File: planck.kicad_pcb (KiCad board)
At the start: 2 copper layers, 113 x 75 mm, 84 parts, among them J1 USB_C_U262-161N-4BVC11, J2 USB_C_U262-161N-4BVC11, SW1 SW_Cherry_MX_1.00u, SW10 SW_Cherry_MX_1.00u, SW11 SW_Cherry_MX_1.00u, SW12 SW_Cherry_MX_1.00u, SW13 SW_Cherry_MX_1.00u, SW14 SW_Cherry_MX_1.00u, SW15 SW_Cherry_MX_1.00u, SW16 SW_Cherry_MX_1.00u, SW17 SW_Cherry_MX_1.00u, SW18 SW_Cherry_MX_1.00u, SW19 SW_Cherry_MX_1.00u, SW2 SW_Cherry_MX_1.00u, SW20 SW_Cherry_MX_1.00u, SW21 SW_Cherry_MX_1.00u, SW22 SW_Cherry_MX_1.00u, SW23 SW_Cherry_MX_1.00u, SW24 SW_Cherry_MX_1.00u, SW25 SW_Push, SW3 SW_Cherry_MX_1.00u, SW4 SW_Cherry_MX_1.00u, SW5 SW_Cherry_MX_1.00u, SW6 SW_Cherry_MX_1.00u, SW7 SW_Cherry_MX_1.00u, SW8 SW_Cherry_MX_1.00u, SW9 SW_Cherry_MX_1.00u, U1 RP2040 ARM Cortex-M0 133MHz, U2 ME6219C33M5G, U3 W25Q16JVUXIQ, Y1 32MHz ±10ppm 20pF SMD3225-4P

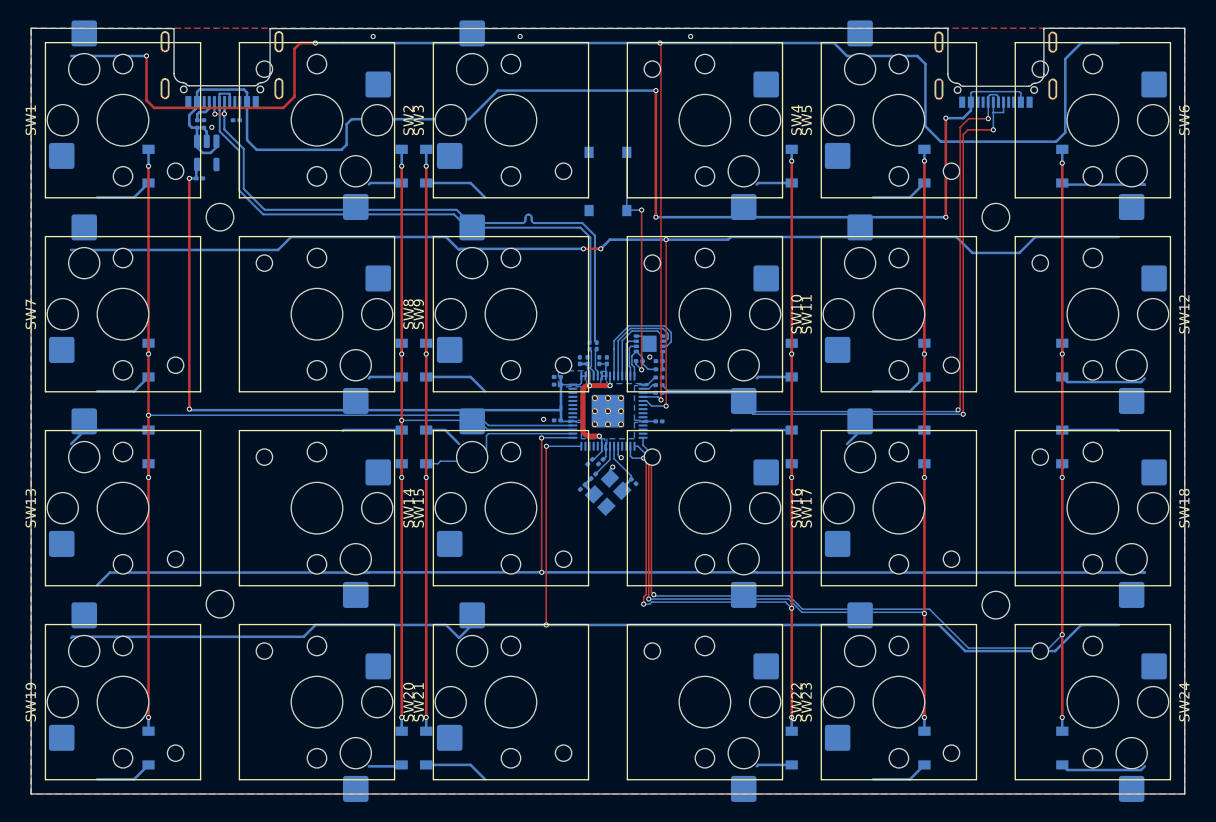
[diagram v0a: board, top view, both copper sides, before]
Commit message: main layouts
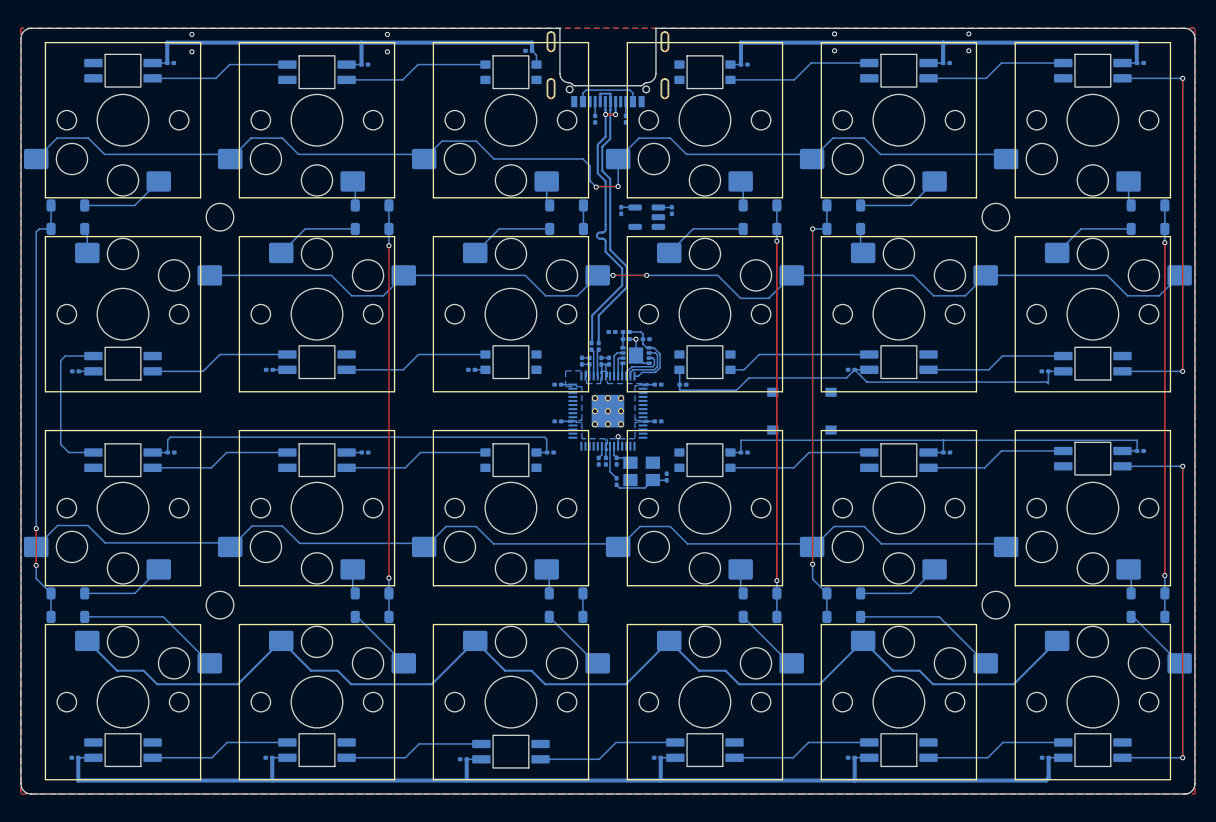
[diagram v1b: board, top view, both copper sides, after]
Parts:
- removed J1: USB_C_U262-161N-4BVC11, josh-connectors:USB_C_TYPE-C-31-M-14
- removed R4, R7: 100Ω ±1% 50mW, Resistor_SMD:R_0201_0603Metric
- added C17: 100nF ±10% 25V 0201, Resistor_SMD:R_0201_0603Metric, B.Cu at (143.8, 131.4)
- added C18: 100nF ±10% 25V 0201, Resistor_SMD:R_0201_0603Metric, B.Cu at (152.3, 101.5)
- added C19: 100nF ±10% 25V 0201, Resistor_SMD:R_0201_0603Metric, B.Cu at (191.2, 101.4)
- added C20: 100nF ±10% 25V 0201, Resistor_SMD:R_0201_0603Metric, B.Cu at (115.2, 63.5)
- added C21: 100nF ±10% 25V 0201, Resistor_SMD:R_0201_0603Metric, B.Cu at (96.2, 63.4)
- added C22: 100nF ±10% 25V 0201, Resistor_SMD:R_0201_0603Metric, B.Cu at (162.8, 93.5)
- added C23: 100nF ±10% 25V 0201, Resistor_SMD:R_0201_0603Metric, B.Cu at (86.8, 93.6)
- added C24: 100nF ±10% 25V 0201, Resistor_SMD:R_0201_0603Metric, B.Cu at (124.8, 131.6)
- added C25: 100nF ±10% 25V 0201, Resistor_SMD:R_0201_0603Metric, B.Cu at (115.2, 101.5)
- added C26: 100nF ±10% 25V 0201, Resistor_SMD:R_0201_0603Metric, B.Cu at (172.2, 101.5)
- added C27: 100nF ±10% 25V 0201, Resistor_SMD:R_0201_0603Metric, B.Cu at (181.8, 93.6)
- added C28: 100nF ±10% 25V 0201, Resistor_SMD:R_0201_0603Metric, B.Cu at (125.7, 93.5)
- added C29: 100nF ±10% 25V 0201, Resistor_SMD:R_0201_0603Metric, B.Cu at (146.3, 94.9)
- added C30: 100nF ±10% 25V 0201, Resistor_SMD:R_0201_0603Metric, B.Cu at (105.8, 93.5)
- added C31: 100nF ±10% 25V 0201, Resistor_SMD:R_0201_0603Metric, B.Cu at (105.8, 131.4)
- added C32: 100nF ±10% 25V 0201, Resistor_SMD:R_0201_0603Metric, B.Cu at (96.2, 101.5)
- added C33: 100nF ±10% 25V 0201, Resistor_SMD:R_0201_0603Metric, B.Cu at (133.4, 101.5)
- added C34: 100nF ±10% 25V 0201, Resistor_SMD:R_0201_0603Metric, B.Cu at (191.2, 63.4)
- added C35: 100nF ±10% 25V 0201, Resistor_SMD:R_0201_0603Metric, B.Cu at (172.2, 63.4)
- added C36: 100nF ±10% 25V 0201, Resistor_SMD:R_0201_0603Metric, B.Cu at (152.3, 63.5)
- added C37: 100nF ±10% 25V 0201, Resistor_SMD:R_0201_0603Metric, B.Cu at (131.2, 62.2)
- added C38: 100nF ±10% 25V 0201, Resistor_SMD:R_0201_0603Metric, B.Cu at (86.8, 131.4)
- added C39: 100nF ±10% 25V 0201, Resistor_SMD:R_0201_0603Metric, B.Cu at (181.8, 131.4)
- added C40: 100nF ±10% 25V 0201, Resistor_SMD:R_0201_0603Metric, B.Cu at (162.8, 131.4)
- added D25: WS2812B, MCU_RaspberryPi_and_Boards:WS2812_6028_REV, F.Cu at (91.5, 64.2)
- added D26: WS2812B, MCU_RaspberryPi_and_Boards:WS2812_6028_REV, F.Cu at (110.5, 64.3)
- added D27: WS2812B, MCU_RaspberryPi_and_Boards:WS2812_6028_REV_S, F.Cu at (129.5, 64.3)
- added D28: WS2812B, MCU_RaspberryPi_and_Boards:WS2812_6028_REV_S, F.Cu at (148.5, 64.3)
- added D29: WS2812B, MCU_RaspberryPi_and_Boards:WS2812_6028_REV, F.Cu at (167.5, 64.2)
- added D30: WS2812B, MCU_RaspberryPi_and_Boards:WS2812_6028_REV, F.Cu at (186.5, 64.2)
- added D31: WS2812B, MCU_RaspberryPi_and_Boards:WS2812_6028_REV, F.Cu at (186.5, 92.8)
- added D32: WS2812B, MCU_RaspberryPi_and_Boards:WS2812_6028_REV, F.Cu at (167.5, 92.7)
- added D33: WS2812B, MCU_RaspberryPi_and_Boards:WS2812_6028_REV_S, F.Cu at (148.5, 92.7)
- added D34: WS2812B, MCU_RaspberryPi_and_Boards:WS2812_6028_REV_S, F.Cu at (129.5, 92.7)
- added D35: WS2812B, MCU_RaspberryPi_and_Boards:WS2812_6028_REV, F.Cu at (110.5, 92.7)
- added D36: WS2812B, MCU_RaspberryPi_and_Boards:WS2812_6028_REV, F.Cu at (91.5, 92.8)
- added D37: WS2812B, MCU_RaspberryPi_and_Boards:WS2812_6028_REV, F.Cu at (91.5, 102.3)
- added D38: WS2812B, MCU_RaspberryPi_and_Boards:WS2812_6028_REV, F.Cu at (110.5, 102.3)
- added D39: WS2812B, MCU_RaspberryPi_and_Boards:WS2812_6028_REV_S, F.Cu at (129.5, 102.3)
- added D40: WS2812B, MCU_RaspberryPi_and_Boards:WS2812_6028_REV_S, F.Cu at (148.5, 102.3)
- added D41: WS2812B, MCU_RaspberryPi_and_Boards:WS2812_6028_REV, F.Cu at (167.5, 102.3)
- added D42: WS2812B, MCU_RaspberryPi_and_Boards:WS2812_6028_REV, F.Cu at (186.5, 102.2)
- added D43: WS2812B, MCU_RaspberryPi_and_Boards:WS2812_6028_REV, F.Cu at (186.5, 130.7)
- added D44: WS2812B, MCU_RaspberryPi_and_Boards:WS2812_6028_REV, F.Cu at (167.5, 130.7)
- added D45: WS2812B, MCU_RaspberryPi_and_Boards:WS2812_6028_REV, F.Cu at (148.5, 130.7)
- added D46: WS2812B, MCU_RaspberryPi_and_Boards:WS2812_6028_REV, F.Cu at (129.5, 130.8)
- added D47: WS2812B, MCU_RaspberryPi_and_Boards:WS2812_6028_REV, F.Cu at (110.5, 130.7)
- added D48: WS2812B, MCU_RaspberryPi_and_Boards:WS2812_6028_REV, F.Cu at (91.5, 130.7)
- SW1, SW10, SW11, SW12, SW13, SW14, SW15, SW16, SW17, SW18, SW19, SW2, SW20, SW21, SW22, SW23, SW24, SW3, SW4, SW5, SW6, SW7, SW8, SW9: value SW_Cherry_MX_1.00u -> SW_Hotswap_Kailh_Choc_V1_1u; footprint Switch_Keyboard_Hotswap_Kailh:SW_Hotswap_Kailh_Choc_V1V2 -> Switch_Keyboard_Kailh:SW_Hotswap_Kailh_Choc_V1
- moved C1 46.9 mm to (145.3, 77.8), turned to -90 degrees
- moved U2 43.6 mm to (142.8, 78.5), turned to 180 degrees
- moved C2 41.4 mm to (140.3, 77.8), turned to -90 degrees
- moved R1 38.7 mm to (137.8, 68.9), turned to -90 degrees
- moved R2 38.2 mm to (140.8, 68.9), turned to -90 degrees
- moved J2 37.8 mm to (139.0, 64.3)
- moved SW25 29.4 mm to (158.0, 97.5), turned to 0 degrees
- moved D15 19.8 mm to (134.9, 115.3), turned to 0 degrees
- moved D9 18.8 mm to (134.9, 79.7), turned to 0 degrees
- moved D21 18.8 mm to (134.9, 117.7), turned to 0 degrees
- moved D18 16.6 mm to (191.9, 115.3), turned to 0 degrees
- moved D13 16.4 mm to (86.1, 115.3), turned to 180 degrees
- moved D17 16.4 mm to (162.1, 115.3), turned to 180 degrees
- moved D12 15.4 mm to (191.9, 79.7), turned to 0 degrees
- moved D24 15.4 mm to (191.9, 117.7), turned to 0 degrees
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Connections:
- D10 pad 1: Net-(D10-Pad1) -> Net-(D10-K)
- D12 pad 1: Net-(D12-Pad1) -> Net-(D12-K)
- D13 pad 1: Net-(D13-Pad1) -> Net-(D13-K)
- D15 pad 1: Net-(D15-Pad1) -> Net-(D15-K)
- D17 pad 1: Net-(D17-Pad1) -> Net-(D17-K)
- D19 pad 1: Net-(D19-Pad1) -> Net-(D19-K)
- D2 pad 1: Net-(D2-Pad1) -> Net-(D2-K)
- D21 pad 1: Net-(D21-Pad1) -> Net-(D21-K)
- D23 pad 1: Net-(D23-Pad1) -> Net-(D23-K)
- D4 pad 1: Net-(D4-Pad1) -> Net-(D4-K)
- D6 pad 1: Net-(D6-Pad1) -> Net-(D6-K)
- D8 pad 1: Net-(D8-Pad1) -> Net-(D8-K)
- SW10 pad 1: r2 -> Net-(D10-K)
- SW10 pad 2: Net-(D10-Pad1) -> r2
- SW12 pad 1: r2 -> Net-(D12-K)
- SW12 pad 2: Net-(D12-Pad1) -> r2
- SW13 pad 1: r3 -> Net-(D13-K)
- SW13 pad 2: Net-(D13-Pad1) -> r3
- SW15 pad 1: r3 -> Net-(D15-K)
- SW15 pad 2: Net-(D15-Pad1) -> r3
- SW17 pad 1: r3 -> Net-(D17-K)
- SW17 pad 2: Net-(D17-Pad1) -> r3
- SW19 pad 1: Net-(D19-Pad1) -> r4
- SW19 pad 2: r4 -> Net-(D19-K)
- SW2 pad 1: r1 -> Net-(D2-K)
- SW2 pad 2: Net-(D2-Pad1) -> r1
- SW21 pad 1: Net-(D21-Pad1) -> r4
- SW21 pad 2: r4 -> Net-(D21-K)
- SW23 pad 1: Net-(D23-Pad1) -> r4
- SW23 pad 2: r4 -> Net-(D23-K)
- SW4 pad 1: r1 -> Net-(D4-K)
- SW4 pad 2: Net-(D4-Pad1) -> r1
- SW6 pad 1: r1 -> Net-(D6-K)
- SW6 pad 2: Net-(D6-Pad1) -> r1
- SW8 pad 1: r2 -> Net-(D8-K)
- SW8 pad 2: Net-(D8-Pad1) -> r2
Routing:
- net /VBUS: track 684.4 -> 356.5 mm, vias 31 -> 0
- net c3: track 76.3 -> 4.60 mm, vias 4 -> 0
- net /V3V3: track 76.6 -> 10.2 mm, vias 2 -> 0
- net c1: track 101.4 -> 42.2 mm, vias 5 -> 2
- net r1: track 165.4 -> 108.0 mm, vias 4 -> 2
- net c5: track 0.00 -> 42.3 mm, vias 0 -> 2
- net Net-(D30-DOUT): track 0.00 -> 40.5 mm, vias 0 -> 2
- net Net-(D42-DOUT): track 0.00 -> 40.3 mm, vias 0 -> 2
- net c6: track 0.00 -> 40.3 mm, vias 0 -> 2
- net c4: track 0.00 -> 40.3 mm, vias 0 -> 2
- net c2: track 76.5 -> 40.3 mm, vias 5 -> 2
- net /D+: track 0.00 -> 29.6 mm, vias 0 -> 2
- net /D-: track 0.00 -> 28.7 mm
- net Net-(R9-Pad1): track 23.9 -> 0.00 mm, vias 2 -> 0
- net r2: track 124.3 -> 103.5 mm, vias 4 -> 2
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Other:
- board size 113 x 75 mm -> 115 x 75 mm
- board text added: "BOOT"
- board text removed: "boot"
